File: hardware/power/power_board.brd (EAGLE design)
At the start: 92 x 92 mm, 72 parts, among them IC1 LM321MF, IC2 LM321MF, J1 FASTON1289_ST, J2 FASTON1289_ST, J3 12v, J4 5v, J5 XT30PW-F, J6 XT30PW-F, J7 XT30PW-F, J8 XT30PW-F, U1 PDQ30-Q24-S5-D, U2 PDQ30-Q24-S12-D

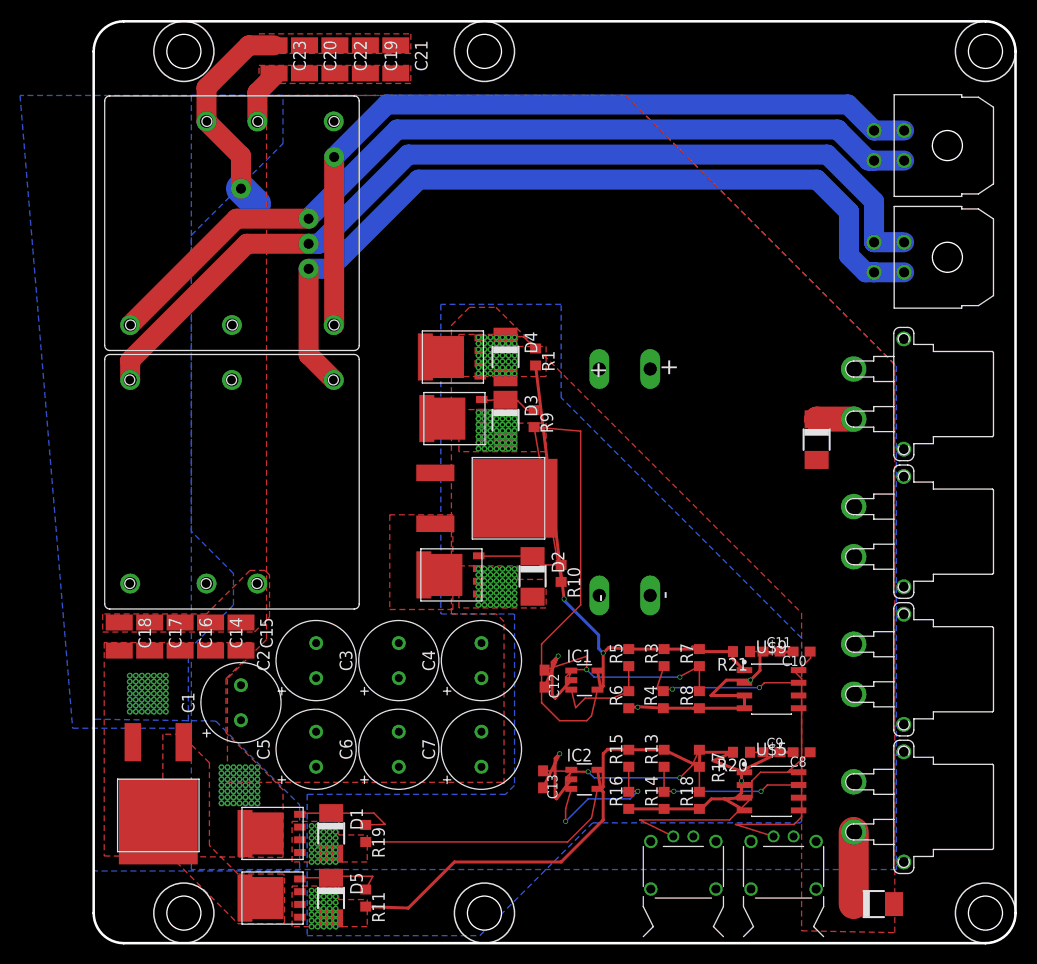
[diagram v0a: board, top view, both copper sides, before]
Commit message: Fixed weird export issue
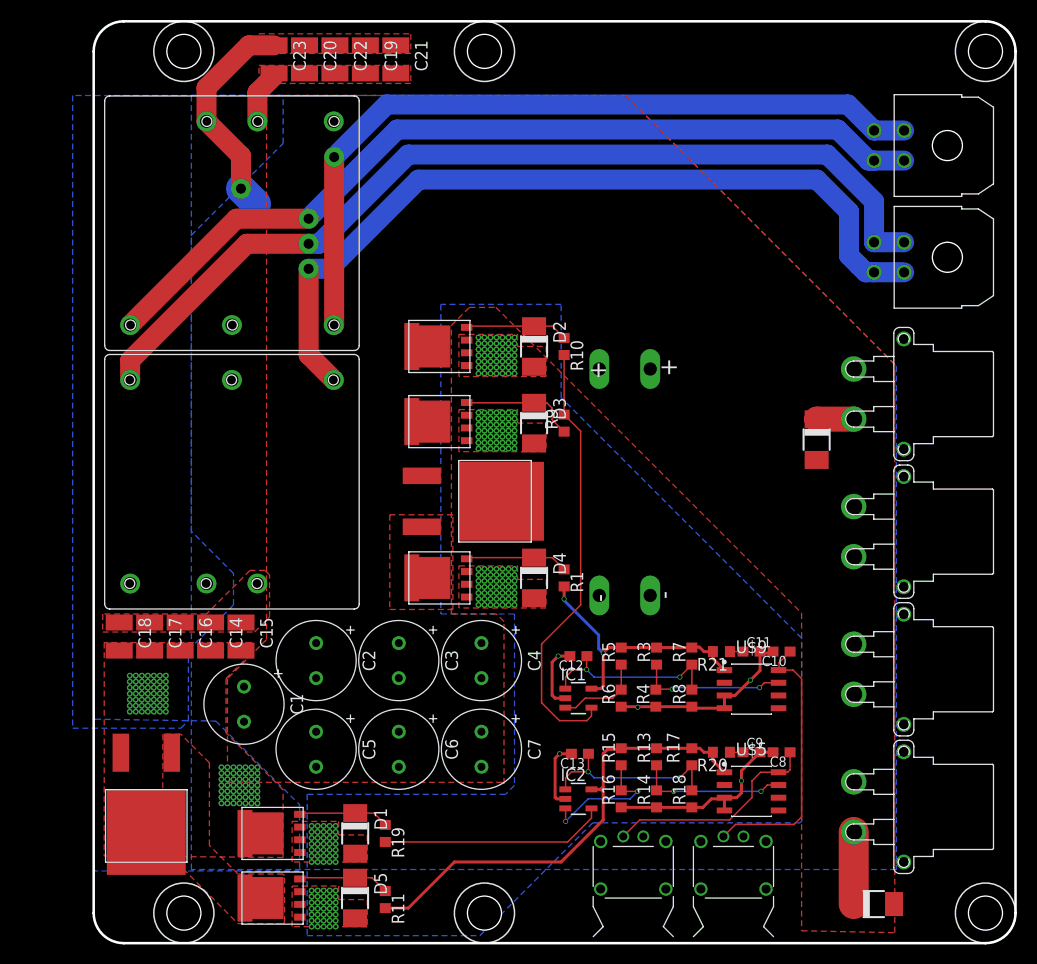
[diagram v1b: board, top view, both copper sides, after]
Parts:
- moved D2 23.0 mm to (44.0, 59.5)
- moved U$2 22.8 mm to (34.5, 59.5)
- moved R10 22.7 mm to (47.0, 59.5)
- moved D4 22.2 mm to (44.0, 36.5)
- moved R1 22.2 mm to (47.0, 36.5)
- moved U$11 22.1 mm to (34.5, 36.5)
- moved U$26 5.00 mm to (53.9, 10.7)
- moved U$27 5.00 mm to (63.9, 10.7)
- moved C13 4.47 mm to (48.5, 18.9), turned to 180 degrees
- moved C12 4.06 mm to (48.4, 28.6), turned to 180 degrees
- moved R9 3.03 mm to (47.0, 51.9), turned to 90 degrees
- moved D3 2.87 mm to (44.0, 51.9)
- moved D1 2.40 mm to (26.1, 10.9)
- moved D5 2.40 mm to (26.1, 4.50)
- moved IC2 2.04 mm to (48.4, 14.4)
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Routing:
- net LEG_12V: track 53.2 -> 26.5 mm
- net BATT_GND: track 75.2 -> 53.0 mm
- net N$6: track 57.7 -> 43.7 mm
- net ISO_12V: track 57.1 -> 46.9 mm
- net N$13: track 27.2 -> 19.1 mm
- net N$5: track 25.5 -> 18.8 mm
- net N$8: track 5.97 -> 11.6 mm
- net N$18: track 26.6 -> 22.1 mm
- net N$14: track 26.5 -> 22.5 mm
- net N$2: track 6.42 -> 10.3 mm
- net N$3: track 18.3 -> 15.1 mm
- net N$12: track 16.5 -> 13.9 mm
- net N$10: track 17.5 -> 15.0 mm
- net N$15: track 11.0 -> 9.09 mm
- net N$9: track 8.71 -> 10.3 mm
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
